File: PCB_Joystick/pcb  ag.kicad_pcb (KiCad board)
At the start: 2 copper layers, 150 x 150 mm, 29 parts, among them J2 Conn_01x05, SW10 SW_Push_LED, SW6 SW_Push_LED, SW7 SW_Push_LED, SW8 SW_Push_LED, SW9 SW_Push_LED, U2 TP4056-42-ESOP8, U3 FS8205A_C2830320, U4 DW01A_C351410, U5 10155435-00011LF

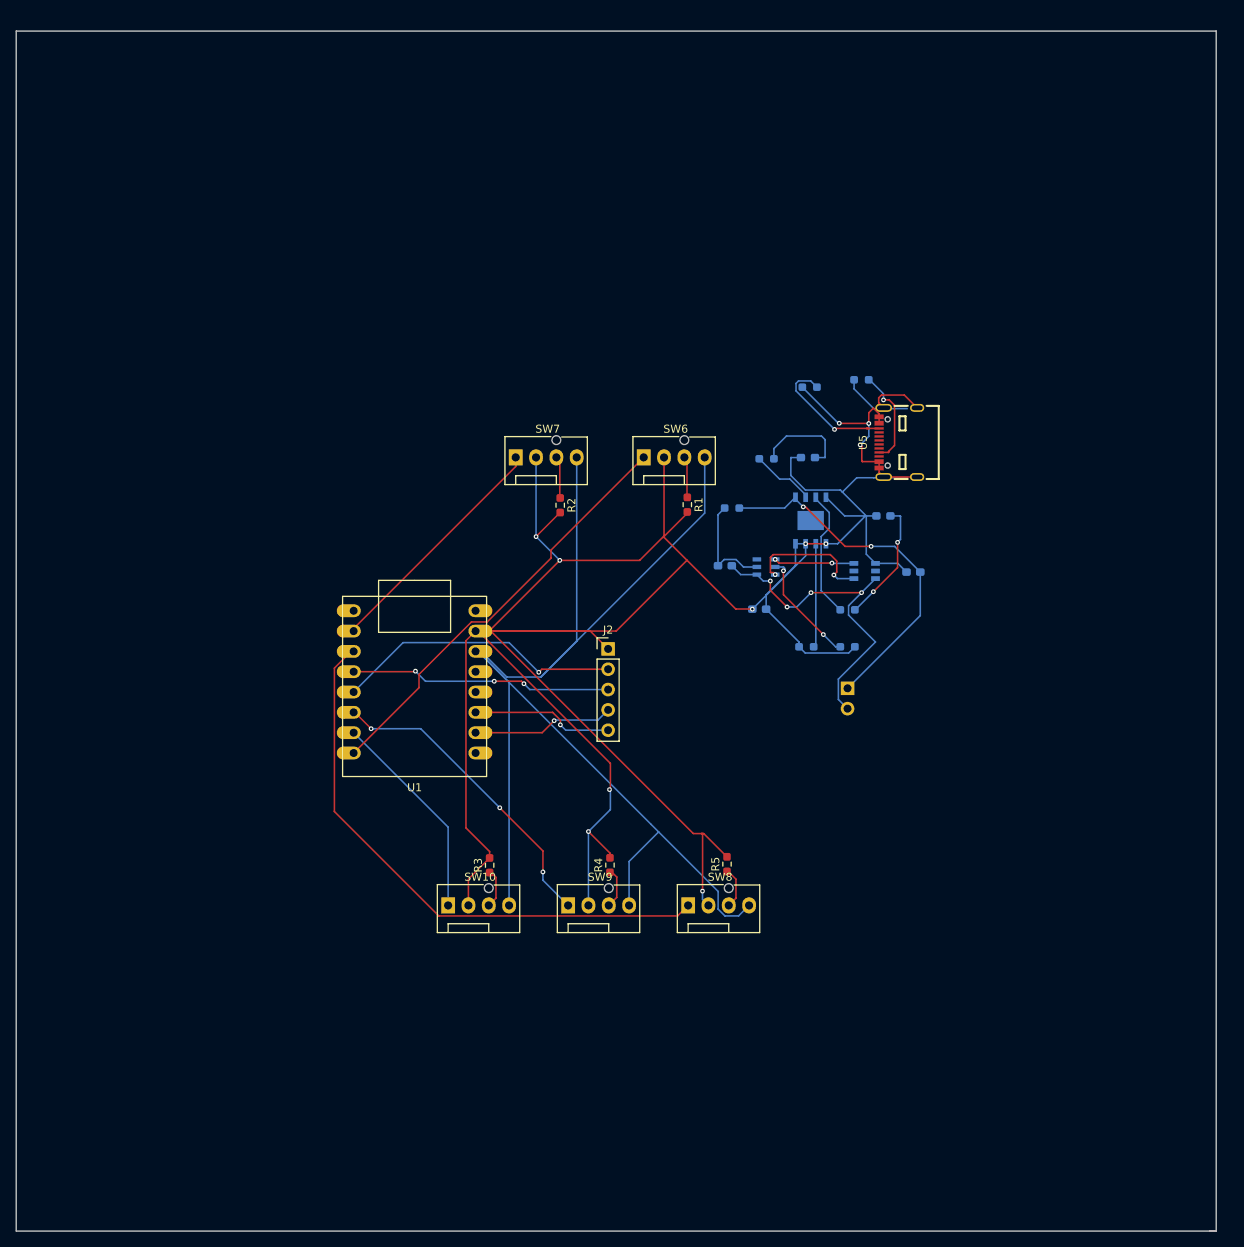
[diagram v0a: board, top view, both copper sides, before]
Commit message: upd
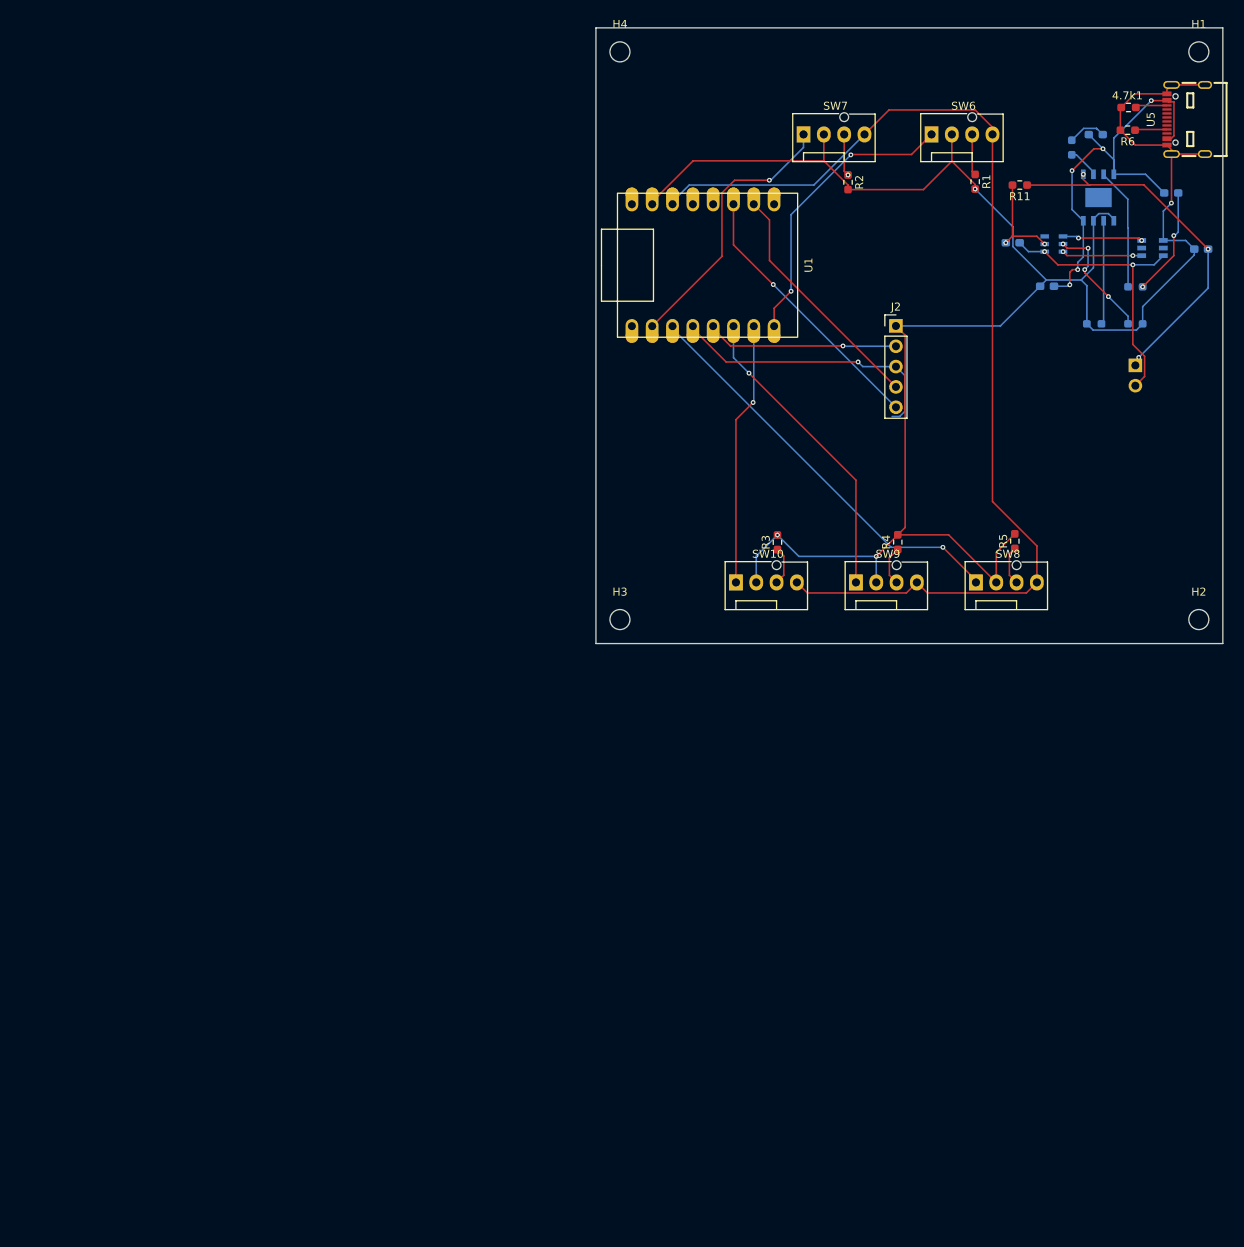
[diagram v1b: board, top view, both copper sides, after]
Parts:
- added H1: MountingHole, MountingHole:MountingHole_2.5mm, F.Cu at (138.3, -16.1)
- added H2: MountingHole, MountingHole:MountingHole_2.5mm, F.Cu at (138.3, 54.8)
- added H3: MountingHole, MountingHole:MountingHole_2.5mm, F.Cu at (66.0, 54.8)
- added H4: MountingHole, MountingHole:MountingHole_2.5mm, F.Cu at (66.0, -16.1)
- 4.7k1, R11, R6: moved to F.Cu
- moved U1 64.5 mm to (77.2, 10.6), turned to 90 degrees
- moved R8 54.5 mm to (122.5, -4.16), turned to -90 degrees
- moved U5 54.1 mm to (136.7, -7.67)
- moved C3 54.1 mm to (115.1, 7.74)
- moved D6 54.1 mm to (125.5, -5.78)
- moved R2 54.1 mm to (94.5, 0.18)
- moved U4 54.1 mm to (120.2, 7.90)
- moved BT1 54.1 mm to (130.4, 23.1)
- moved C1 54.1 mm to (119.4, 13.2)
- moved D7 54.1 mm to (134.9, 1.51)
- moved J2 54.1 mm to (100.5, 18.1)
- moved R1 54.1 mm to (110.4, 0.11)
- moved R10 54.1 mm to (130.4, 17.9)
- moved R11 54.1 mm to (116.0, 0.53)
- moved R12 54.1 mm to (125.3, 17.9)
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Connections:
- C1 pad 1: GND -> Net-(D6-A)
- D6 pad 2: GND -> Net-(D6-A)
- D7 pad 2: GND -> Net-(D6-A)
- U2 pad 4: GND -> Net-(D6-A)
- U2 pad 8: GND -> Net-(D6-A)
- U5 pad A4B9: GND -> Net-(D6-A)
- U5 pad A6: /D+ -> unconnected-(U5-Dp1-PadA6)
- U5 pad A7: /D- -> unconnected-(U5-Dn1-PadA7)
- U5 pad B4A9: GND -> Net-(D6-A)
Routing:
- net GND: track 391.4 -> 251.2 mm, vias 11 -> 4
- net Net-(D6-A): track 0.00 -> 56.1 mm, vias 0 -> 5
- net +3V3: track 168.5 -> 137.3 mm
- net /3button.gpio7: track 71.4 -> 51.5 mm, vias 0 -> 1
- net /1button.gpio5: track 53.1 -> 36.6 mm, vias 0 -> 2
- net /5.2button.gpio2: track 17.8 -> 33.8 mm
- net Net-(U5-CC2): track 16.7 -> 4.00 mm, vias 1 -> 0
- net /4.2button.gpio1: track 17.8 -> 30.2 mm, vias 1 -> 0
- net /2.2button.gpio9: track 36.1 -> 24.1 mm
- net Net-(U5-CC1): track 12.6 -> 4.13 mm, vias 1 -> 0
- net Net-(D6-K): track 12.0 -> 4.94 mm
- net /5button.gpio20: track 26.5 -> 33.0 mm, vias 0 -> 1
- net Net-(U3-G2): track 16.1 -> 10.0 mm
- net Net-(BT1--): track 41.5 -> 35.8 mm, vias 4 -> 2
- net Net-(U2-~{STDBY}): track 7.96 -> 3.89 mm
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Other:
- board size 150 x 150 mm -> 78.4 x 77 mm
